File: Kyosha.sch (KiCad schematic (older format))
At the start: 64 parts, among them SW1 SW_PUSH, SW10 SW_PUSH, SW11 SW_PUSH, SW12 SW_PUSH, SW13 SW_PUSH, SW14 SW_PUSH, SW15 SW_PUSH, SW16 SW_PUSH, SW17 SW_PUSH, SW18 SW_PUSH, SW19 SW_PUSH, SW2 SW_PUSH, SW20 SW_PUSH, SW21 SW_PUSH, SW22 SW_PUSH, SW23 SW_PUSH, SW24 SW_PUSH, SW25 SW_PUSH, SW26 SW_PUSH, SW27 SW_PUSH, SW28 SW_PUSH, SW29 SW_PUSH, SW3 SW_PUSH, SW30 SW_PUSH, SW31 SW_PUSH, SW32 SW_PUSH, SW4 SW_PUSH, SW5 SW_PUSH, SW6 SW_PUSH, SW7 SW_PUSH, SW8 SW_PUSH, SW9 SW_PUSH, U1 ProMicro

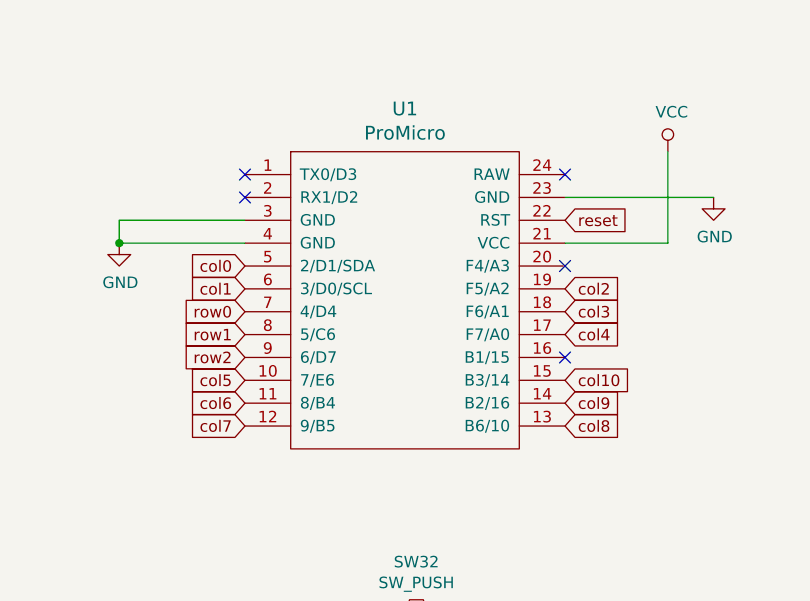
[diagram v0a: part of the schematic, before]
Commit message: pcb first pass
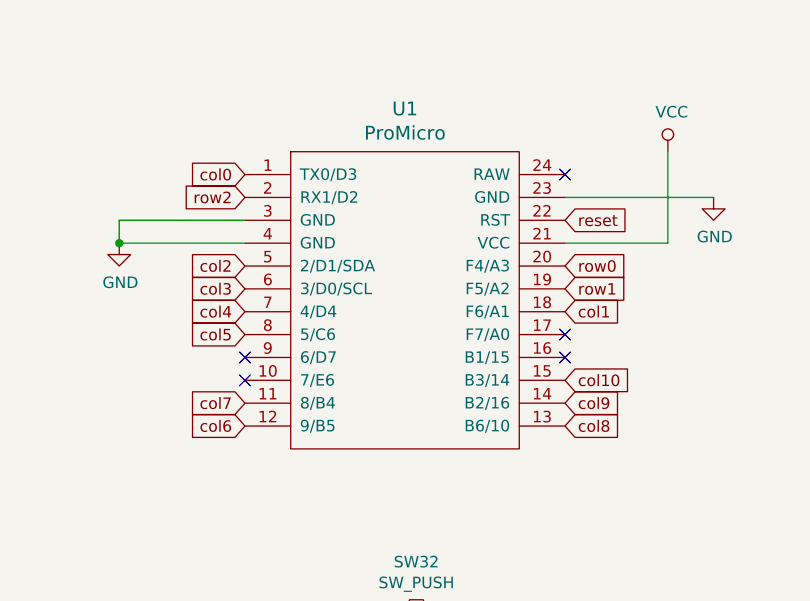
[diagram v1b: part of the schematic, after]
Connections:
- net col0: now also U1.1 (TX0/D3); no longer U1.5 (2/D1/SDA)
- net col1: now also U1.18 (F6/A1); no longer U1.6 (3/D0/SCL)
- net col2: now also U1.5 (2/D1/SDA); no longer U1.19 (F5/A2)
- net col3: now also U1.6 (3/D0/SCL); no longer U1.18 (F6/A1)
- net col4: now also U1.7 (4/D4); no longer U1.17 (F7/A0)
- net col5: now also U1.8 (5/C6); no longer U1.10 (7/E6)
- net col6: now also U1.12 (9/B5); no longer U1.11 (8/B4)
- net col7: now also U1.11 (8/B4); no longer U1.12 (9/B5)
- net row0: now also U1.20 (F4/A3); no longer U1.7 (4/D4)
- net row1: now also U1.19 (F5/A2); no longer U1.8 (5/C6)
- net row2: now also U1.2 (RX1/D2); no longer U1.9 (6/D7)
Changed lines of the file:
@@
 EESchema Schematic File Version 4
+LIBS:Kyosha-cache
 EELAYER 29 0
 EELAYER END
@@
 reset
 NoConn ~ 5850 4100
+Text GLabel 5850 4500 2    50   Input ~ 0
+row0
+Text GLabel 5850 4600 2    50   Input ~ 0
+row1
+Text GLabel 4450 4200 0    50   Input ~ 0
+row2
+Text GLabel 4450 4100 0    50   Input ~ 0
+col0
+Text GLabel 5850 4700 2    50   Input ~ 0
+col1
+Text GLabel 4450 4500 0    50   Input ~ 0
+col2
+Text GLabel 4450 4600 0    50   Input ~ 0
+col3
 Text GLabel 4450 4700 0    50   Input ~ 0
-row0
+col4
 Text GLabel 4450 4800 0    50   Input ~ 0
-row1
-Text GLabel 4450 4900 0    50   Input ~ 0
-row2
-Text GLabel 4450 4500 0    50   Input ~ 0
-col0
-Text GLabel 4450 4600 0    50   Input ~ 0
-col1
-Text GLabel 5850 4600 2    50   Input ~ 0
-col2
-Text GLabel 5850 4700 2    50   Input ~ 0
-col3
-Text GLabel 5850 4800 2    50   Input ~ 0
-col4
-Text GLabel 4450 5000 0    50   Input ~ 0
 col5
+Text GLabel 4450 5100 0    50   Input ~ 0
+col7
 Text GLabel 4450 5200 0    50   Input ~ 0
-col7
-Text GLabel 4450 5100 0    50   Input ~ 0
 col6
 Text GLabel 5850 5000 2    50   Input ~ 0
@@
 Text GLabel 5850 5200 2    50   Input ~ 0
 col8
-NoConn ~ 5850 4500
-NoConn ~ 4450 4200
-NoConn ~ 4450 4100
 NoConn ~ 5850 4900
+NoConn ~ 5850 4800
+NoConn ~ 4450 4900
+NoConn ~ 4450 5000
 $EndSCHEMATC
